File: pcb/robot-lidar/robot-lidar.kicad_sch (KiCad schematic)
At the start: 33 parts, among them J12 Conn_02x20_Odd_Even, J2 YLIDAR X4, J3 Jack-DC, J5 Conn_01x02, J5 Conn_02x03_Odd_Even, J6 Conn_01x02, J7 Conn_01x02, J7 Conn_ARM_SWD_TagConnect_TC2030, J8 Conn_01x02, U1 STM32F103C8Tx, U2 LM317-3.3_SOT-223, U2 MPU-6050, U4 MX1508, U5 MX1508, Y1 Crystal

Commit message: PCA9685
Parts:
- removed C14, C15: 0.1uF, Capacitor_SMD:C_0603_1608Metric, symbol Device:C_Small
- removed J5: Conn_02x03_Odd_Even, Connector_PinHeader_2.54mm:PinHeader_2x03_P2.54mm_Vertical_SMD, symbol Connector_Generic:Conn_02x03_Odd_Even
- removed J7: Conn_ARM_SWD_TagConnect_TC2030, Connector_PinHeader_2.54mm:PinHeader_1x06_P2.54mm_Vertical, symbol Connector:Conn_ARM_SWD_TagConnect_TC2030
- removed R6, R7, R8, R9: 10k, Resistor_SMD:R_0603_1608Metric, symbol Device:R_Small
- removed U1: STM32F103C8Tx, Package_QFP:LQFP-48_7x7mm_P0.5mm, symbol MCU_ST_STM32F1:STM32F103C8Tx
- removed Y1: Crystal, Crystal:Crystal_SMD_HC49-SD, symbol Device:Crystal
- added R1: R_Small, Resistor_SMD:R_0603_1608Metric, symbol Device:R_Small
- added U1: PCA9635, Package_SO:TSSOP-28_4.4x9.7mm_P0.65mm, symbol Driver_LED:PCA9635
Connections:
- net +5V: now also U1.28 (VDD)
- net GND: now also R1.1, U1.1 (A0), U1.14 (VSS), U1.2 (A1), U1.24 (A5), U1.25 (A6), U1.3 (A2), U1.4 (A3), U1.5 (A4)
- net MOTOR_1_A: now also U1.6 (LED0)
- net MOTOR_1_B: now also U1.7 (LED1)
- net MOTOR_2_A: now also U1.8 (LED2)
- net MOTOR_2_B: now also U1.9 (LED3)
- net MOTOR_3_A: now also U1.10 (LED4)
- net MOTOR_3_B: now also U1.11 (LED5)
- net MOTOR_4_A: now also U1.12 (LED6)
- net MOTOR_4_B: now also U1.13 (LED7)
- net SCL: now also U1.26 (SCL)
- net SDA: now also U1.27 (SDA)
- new net: R1.2, U1.23 (~{OE})
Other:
- moved on the sheet: C1, C2, C3, R1, R2, U2

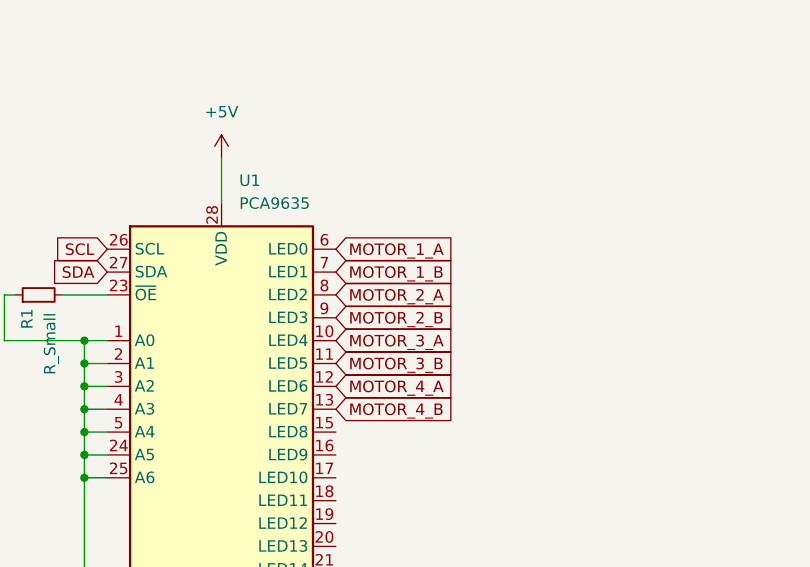
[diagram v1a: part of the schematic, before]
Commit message: wiring pca
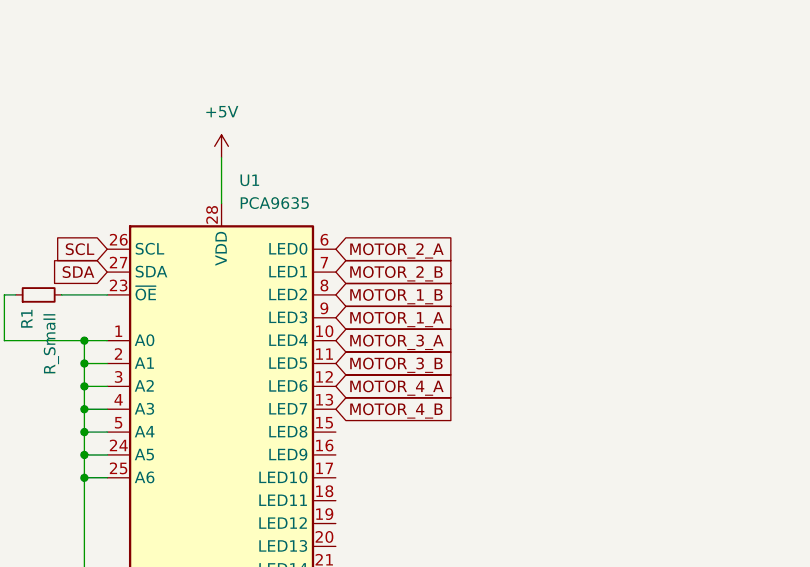
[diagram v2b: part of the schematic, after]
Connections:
- net MOTOR_1_A: now also U1.9 (LED3); no longer U1.6 (LED0)
- net MOTOR_1_B: now also U1.8 (LED2); no longer U1.7 (LED1)
- net MOTOR_2_A: now also U1.6 (LED0); no longer U1.8 (LED2)
- net MOTOR_2_B: now also U1.7 (LED1); no longer U1.9 (LED3)
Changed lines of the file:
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@@
+    )
+  )
+  (global_label "MOTOR_2_A" (shape input) (at 115.57 54.61 0) (fields_autoplaced)
+    (effects (font (size 1.27 1.27)) (justify left))
+    (property "Intersheetrefs" "${INTERSHEET_REFS}" (at 129.0591 54.61 0)
+      (effects (font (size 1.27 1.27)) (justify left) hide)
     )
   )
@@
     )
   )
+  (global_label "MOTOR_1_A" (shape input) (at 115.57 62.23 0) (fields_autoplaced)
+    (effects (font (size 1.27 1.27)) (justify left))
+    (property "Intersheetrefs" "${INTERSHEET_REFS}" (at 129.0591 62.23 0)
+      (effects (font (size 1.27 1.27)) (justify left) hide)
+    )
+  )
   (global_label "M_EN" (shape input) (at 48.26 190.5 180) (fields_autoplaced)
     (effects (font (size 1.27 1.27)) (justify right))
@@
     )
   )
-  (global_label "MOTOR_1_A" (shape input) (at 115.57 54.61 0) (fields_autoplaced)
-    (effects (font (size 1.27 1.27)) (justify left))
-    (property "Intersheetrefs" "${INTERSHEET_REFS}" (at 129.0591 54.61 0)
-      (effects (font (size 1.27 1.27)) (justify left) hide)
-    )
-  )
   (global_label "MOTOR_4_A" (shape input) (at 214.63 147.32 180) (fields_autoplaced)
     (effects (font (size 1.27 1.27)) (justify right))
@@
     )
   )
-  (global_label "MOTOR_1_B" (shape input) (at 115.57 57.15 0) (fields_autoplaced)
+  (global_label "MOTOR_2_B" (shape input) (at 115.57 57.15 0) (fields_autoplaced)
     (effects (font (size 1.27 1.27)) (justify left))
     (property "Intersheetrefs" "${INTERSHEET_REFS}" (at 129.2405 57.15 0)
@@
     )
   )
-  (global_label "MOTOR_2_A" (shape input) (at 115.57 59.69 0) (fields_autoplaced)
+  (global_label "MOTOR_1_B" (shape input) (at 115.57 59.69 0) (fields_autoplaced)
     (effects (font (size 1.27 1.27)) (justify left))
-    (property "Intersheetrefs" "${INTERSHEET_REFS}" (at 129.0591 59.69 0)
+    (property "Intersheetrefs" "${INTERSHEET_REFS}" (at 129.2405 59.69 0)
       (effects (font (size 1.27 1.27)) (justify left) hide)
     )
@@
     )
   )
-  (global_label "MOTOR_2_B" (shape input) (at 115.57 62.23 0) (fields_autoplaced)
-    (effects (font (size 1.27 1.27)) (justify left))
-    (property "Intersheetrefs" "${INTERSHEET_REFS}" (at 129.2405 62.23 0)
-      (effects (font (size 1.27 1.27)) (justify left) hide)
-    )
-  )
